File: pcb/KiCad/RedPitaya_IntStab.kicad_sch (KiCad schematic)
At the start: 28 parts, among them J1 C64AC, J16 Hold_2, J4 Hold_1

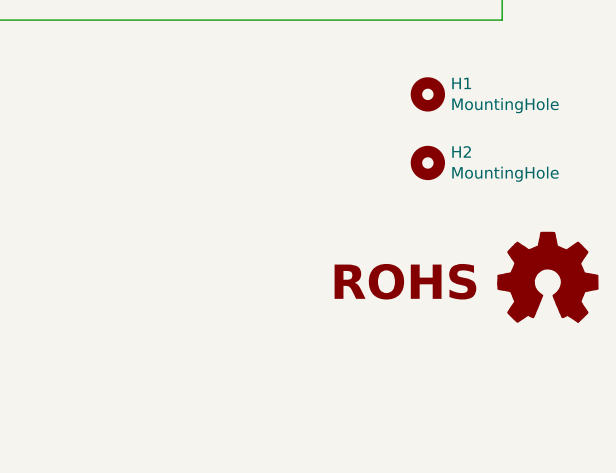
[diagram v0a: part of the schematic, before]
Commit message: More logo updates
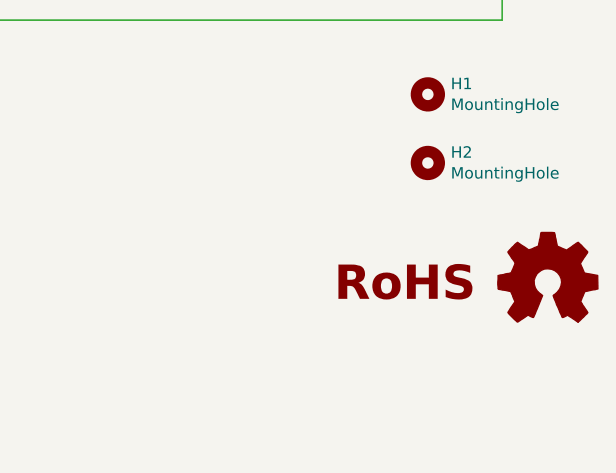
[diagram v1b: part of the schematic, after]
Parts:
- LOGO1, LOGO3: now left out of the parts list
- LOGO2: value Logo_ROHS -> Logo_RoHS; symbol Custom_logos:Logo_ROHS -> Custom_logos:Logo_RoHS; now left out of the parts list
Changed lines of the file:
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@@
   )
   (symbol (lib_id "Custom_logos:Logo_APQ") (at 173.99 171.45 0) (unit 1)
-    (in_bom yes) (on_board yes) (dnp no)
+    (in_bom no) (on_board yes) (dnp no)
     (property "Reference" "LOGO1" (at 180.34 164.465 0)
       (effects (font (size 1.27 1.27)) hide)
@@
       (effects (font (size 1.27 1.27)) hide)
     )
+    (property "MFN" "" (at 173.99 171.45 0)
+      (effects (font (size 1.27 1.27)) hide)
+    )
+    (property "PN" "" (at 173.99 171.45 0)
+      (effects (font (size 1.27 1.27)) hide)
+    )
+    (property "Sim.Enable" "0" (at 173.99 171.45 0)
+      (effects (font (size 1.27 1.27)) hide)
+    )
     (instances
       (project "RedPitaya_IntStab"
@@
   )
   (symbol (lib_id "Graphic:Logo_Open_Hardware_Small") (at 278.13 172.72 0) (unit 1)
-    (in_bom yes) (on_board yes) (dnp no)
+    (in_bom no) (on_board yes) (dnp no)
     (property "Reference" "LOGO3" (at 278.13 165.735 0)
       (effects (font (size 1.27 1.27)) hide)
@@
       (effects (font (size 1.27 1.27)) hide)
     )
+    (property "MFN" "" (at 278.13 172.72 0)
+      (effects (font (size 1.27 1.27)) hide)
+    )
+    (property "PN" "" (at 278.13 172.72 0)
+      (effects (font (size 1.27 1.27)) hide)
+    )
+    (property "Sim.Enable" "0" (at 278.13 172.72 0)
+      (effects (font (size 1.27 1.27)) hide)
+    )
     (instances
       (project "RedPitaya_IntStab"
@@
     )
   )
-  (symbol (lib_id "Custom_logos:Logo_ROHS") (at 248.92 172.72 0) (unit 1)
-    (in_bom yes) (on_board yes) (dnp no)
+  (symbol (lib_id "Custom_logos:Logo_RoHS") (at 248.92 172.72 0) (unit 1)
+    (in_bom no) (on_board yes) (dnp no)
     (property "Reference" "LOGO2" (at 255.27 165.735 0)
       (effects (font (size 1.27 1.27)) hide)
     )
-    (property "Value" "Logo_ROHS" (at 255.27 179.07 0)
+    (property "Value" "Logo_RoHS" (at 255.27 179.07 0)
       (effects (font (size 1.27 1.27)) hide)
     )
-    (property "Footprint" "Symbol:RoHS-Logo_6mm_SilkScreen" (at 262.255 168.1734 0)
+    (property "Footprint" "Symbol:RoHS-Logo_6mm_SilkScreen" (at 256.54 172.72 0)
       (effects (font (size 1.27 1.27)) hide)
     )
@@
       (effects (font (size 1.27 1.27)) hide)
     )
+    (property "MFN" "" (at 248.92 172.72 0)
+      (effects (font (size 1.27 1.27)) hide)
+    )
+    (property "PN" "" (at 248.92 172.72 0)
+      (effects (font (size 1.27 1.27)) hide)
+    )
+    (property "Sim.Enable" "0" (at 248.92 172.72 0)
+      (effects (font (size 1.27 1.27)) hide)
+    )

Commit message: Fixed solder jumpers
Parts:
- JP10, JP11, JP12, JP13, JP14, JP15, JP3, JP4, JP5, JP6, JP7, JP8, JP9: footprint Jumper:SolderJumper-2_P1.3mm_Open_RoundedPad1.0x1.5mm -> Jumper:SolderJumper-2_P1.3mm_Bridged_RoundedPad1.0x1.5mm
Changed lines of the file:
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@@
       (effects (font (size 1.27 1.27)))
     )
-    (property "Footprint" "Jumper:SolderJumper-2_P1.3mm_Open_RoundedPad1.0x1.5mm" (at 19.05 171.45 0)
+    (property "Footprint" "Jumper:SolderJumper-2_P1.3mm_Bridged_RoundedPad1.0x1.5mm" (at 19.05 171.45 0)
       (effects (font (size 1.27 1.27)) hide)
     )
@@
       (effects (font (size 1.27 1.27)) hide)
     )
+    (property "MFN" "" (at 19.05 171.45 0)
+      (effects (font (size 1.27 1.27)) hide)
+    )
+    (property "PN" "" (at 19.05 171.45 0)
+      (effects (font (size 1.27 1.27)) hide)
+    )
     (pin "1")
     (pin "2")
@@
       (effects (font (size 1.27 1.27)))
     )
-    (property "Footprint" "Jumper:SolderJumper-2_P1.3mm_Open_RoundedPad1.0x1.5mm" (at 49.53 187.96 0)
+    (property "Footprint" "Jumper:SolderJumper-2_P1.3mm_Bridged_RoundedPad1.0x1.5mm" (at 49.53 187.96 0)
       (effects (font (size 1.27 1.27)) hide)
     )
@@
       (effects (font (size 1.27 1.27)) hide)
     )
+    (property "MFN" "" (at 49.53 187.96 0)
+      (effects (font (size 1.27 1.27)) hide)
+    )
+    (property "PN" "" (at 49.53 187.96 0)
+      (effects (font (size 1.27 1.27)) hide)
+    )
     (pin "1")
     (pin "2")
@@
       (effects (font (size 1.27 1.27)))
     )
-    (property "Footprint" "Jumper:SolderJumper-2_P1.3mm_Open_RoundedPad1.0x1.5mm" (at 19.05 144.78 0)
+    (property "Footprint" "Jumper:SolderJumper-2_P1.3mm_Bridged_RoundedPad1.0x1.5mm" (at 19.05 144.78 0)
       (effects (font (size 1.27 1.27)) hide)
     )
@@
       (effects (font (size 1.27 1.27)) hide)
     )
+    (property "MFN" "" (at 19.05 144.78 0)
+      (effects (font (size 1.27 1.27)) hide)
+    )
+    (property "PN" "" (at 19.05 144.78 0)
+      (effects (font (size 1.27 1.27)) hide)
+    )
     (pin "1")
     (pin "2")
@@
       (effects (font (size 1.27 1.27)))
     )
-    (property "Footprint" "Jumper:SolderJumper-2_P1.3mm_Open_RoundedPad1.0x1.5mm" (at 19.05 129.54 0)
+    (property "Footprint" "Jumper:SolderJumper-2_P1.3mm_Bridged_RoundedPad1.0x1.5mm" (at 19.05 129.54 0)
       (effects (font (size 1.27 1.27)) hide)
     )
@@
       (effects (font (size 1.27 1.27)) hide)
     )
+    (property "MFN" "" (at 19.05 129.54 0)
+      (effects (font (size 1.27 1.27)) hide)
+    )
+    (property "PN" "" (at 19.05 129.54 0)
+      (effects (font (size 1.27 1.27)) hide)
+    )
     (pin "1")
     (pin "2")
@@
       (effects (font (size 1.27 1.27)))
     )
-    (property "Footprint" "Jumper:SolderJumper-2_P1.3mm_Open_RoundedPad1.0x1.5mm" (at 50.8 133.35 0)
+    (property "Footprint" "Jumper:SolderJumper-2_P1.3mm_Bridged_RoundedPad1.0x1.5mm" (at 50.8 133.35 0)
       (effects (font (size 1.27 1.27)) hide)
     )
@@
       (effects (font (size 1.27 1.27)) hide)
     )
+    (property "MFN" "" (at 50.8 133.35 0)
+      (effects (font (size 1.27 1.27)) hide)
+    )
+    (property "PN" "" (at 50.8 133.35 0)
+      (effects (font (size 1.27 1.27)) hide)
+    )
     (pin "1")
     (pin "2")
@@
       (effects (font (size 1.27 1.27)))
     )
-    (property "Footprint" "Jumper:SolderJumper-2_P1.3mm_Open_RoundedPad1.0x1.5mm" (at 19.05 180.34 0)
+    (property "Footprint" "Jumper:SolderJumper-2_P1.3mm_Bridged_RoundedPad1.0x1.5mm" (at 19.05 180.34 0)
       (effects (font (size 1.27 1.27)) hide)
     )
@@
       (effects (font (size 1.27 1.27)) hide)
     )
+    (property "MFN" "" (at 19.05 180.34 0)
+      (effects (font (size 1.27 1.27)) hide)
+    )
+    (property "PN" "" (at 19.05 180.34 0)
+      (effects (font (size 1.27 1.27)) hide)
+    )
     (pin "1")
     (pin "2")
@@
       (effects (font (size 1.27 1.27)))
     )
-    (property "Footprint" "Jumper:SolderJumper-2_P1.3mm_Open_RoundedPad1.0x1.5mm" (at 50.8 124.46 0)
+    (property "Footprint" "Jumper:SolderJumper-2_P1.3mm_Bridged_RoundedPad1.0x1.5mm" (at 50.8 124.46 0)
       (effects (font (size 1.27 1.27)) hide)
     )
@@
       (effects (font (size 1.27 1.27)) hide)
     )
+    (property "MFN" "" (at 50.8 124.46 0)
+      (effects (font (size 1.27 1.27)) hide)
+    )
+    (property "PN" "" (at 50.8 124.46 0)
+      (effects (font (size 1.27 1.27)) hide)
+    )
     (pin "1")
     (pin "2")
@@
       (effects (font (size 1.27 1.27)))
     )
-    (property "Footprint" "Jumper:SolderJumper-2_P1.3mm_Open_RoundedPad1.0x1.5mm" (at 19.05 137.16 0)
+    (property "Footprint" "Jumper:SolderJumper-2_P1.3mm_Bridged_RoundedPad1.0x1.5mm" (at 19.05 137.16 0)
       (effects (font (size 1.27 1.27)) hide)
     )
@@
       (effects (font (size 1.27 1.27)) hide)
     )
+    (property "MFN" "" (at 19.05 137.16 0)
+      (effects (font (size 1.27 1.27)) hide)
+    )
+    (property "PN" "" (at 19.05 137.16 0)
+      (effects (font (size 1.27 1.27)) hide)
+    )
     (pin "1")
     (pin "2")
@@
       (effects (font (size 1.27 1.27)))
     )
-    (property "Footprint" "Jumper:SolderJumper-2_P1.3mm_Open_RoundedPad1.0x1.5mm" (at 19.05 153.67 0)
+    (property "Footprint" "Jumper:SolderJumper-2_P1.3mm_Bridged_RoundedPad1.0x1.5mm" (at 19.05 153.67 0)
       (effects (font (size 1.27 1.27)) hide)
     )
@@
     )
     (property "Config" "DNF" (at 19.05 153.67 0)
+      (effects (font (size 1.27 1.27)) hide)
+    )
+    (property "MFN" "" (at 19.05 153.67 0)
+      (effects (font (size 1.27 1.27)) hide)
+    )
+    (property "PN" "" (at 19.05 153.67 0)
       (effects (font (size 1.27 1.27)) hide)
     )
@@
       (effects (font (size 1.27 1.27)))
     )
-    (property "Footprint" "Jumper:SolderJumper-2_P1.3mm_Open_RoundedPad1.0x1.5mm" (at 49.53 171.45 0)
+    (property "Footprint" "Jumper:SolderJumper-2_P1.3mm_Bridged_RoundedPad1.0x1.5mm" (at 49.53 171.45 0)
       (effects (font (size 1.27 1.27)) hide)
     )
@@
       (effects (font (size 1.27 1.27)) hide)
     )
+    (property "MFN" "" (at 49.53 171.45 0)
+      (effects (font (size 1.27 1.27)) hide)
+    )
+    (property "PN" "" (at 49.53 171.45 0)
+      (effects (font (size 1.27 1.27)) hide)
+    )
     (pin "1")
     (pin "2")
@@
       (effects (font (size 1.27 1.27)))
     )
-    (property "Footprint" "Jumper:SolderJumper-2_P1.3mm_Open_RoundedPad1.0x1.5mm" (at 19.05 121.92 0)
+    (property "Footprint" "Jumper:SolderJumper-2_P1.3mm_Bridged_RoundedPad1.0x1.5mm" (at 19.05 121.92 0)
       (effects (font (size 1.27 1.27)) hide)
     )
@@
       (effects (font (size 1.27 1.27)) hide)
     )
+    (property "MFN" "" (at 19.05 121.92 0)
+      (effects (font (size 1.27 1.27)) hide)
+    )
+    (property "PN" "" (at 19.05 121.92 0)
+      (effects (font (size 1.27 1.27)) hide)
+    )
     (pin "1")
     (pin "2")
@@
       (effects (font (size 1.27 1.27)))
     )
-    (property "Footprint" "Jumper:SolderJumper-2_P1.3mm_Open_RoundedPad1.0x1.5mm" (at 19.05 162.56 0)
+    (property "Footprint" "Jumper:SolderJumper-2_P1.3mm_Bridged_RoundedPad1.0x1.5mm" (at 19.05 162.56 0)
       (effects (font (size 1.27 1.27)) hide)
     )
@@
       (effects (font (size 1.27 1.27)) hide)
     )
+    (property "MFN" "" (at 19.05 162.56 0)
+      (effects (font (size 1.27 1.27)) hide)
+    )
+    (property "PN" "" (at 19.05 162.56 0)
+      (effects (font (size 1.27 1.27)) hide)
+    )
     (pin "1")
     (pin "2")
@@
       (effects (font (size 1.27 1.27)))
     )
-    (property "Footprint" "Jumper:SolderJumper-2_P1.3mm_Open_RoundedPad1.0x1.5mm" (at 50.8 116.84 0)
+    (property "Footprint" "Jumper:SolderJumper-2_P1.3mm_Bridged_RoundedPad1.0x1.5mm" (at 50.8 116.84 0)
       (effects (font (size 1.27 1.27)) hide)
     )
@@
       (effects (font (size 1.27 1.27)) hide)
     )
+    (property "MFN" "" (at 50.8 116.84 0)
+      (effects (font (size 1.27 1.27)) hide)
+    )
+    (property "PN" "" (at 50.8 116.84 0)
+      (effects (font (size 1.27 1.27)) hide)
+    )

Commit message: Fixed logos on the schematic
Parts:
- LOGO1, LOGO2, LOGO3: Config DNF -> (none)
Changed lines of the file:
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@@
-      (effects (font (size 1.27 1.27)) hide)
-    )
-    (property "Config" "DNF" (at 173.99 171.45 0)
       (effects (font (size 1.27 1.27)) hide)
     )
@@
       (effects (font (size 1.27 1.27)) hide)
     )
-    (property "Config" "DNF" (at 278.13 172.72 0)
-      (effects (font (size 1.27 1.27)) hide)
-    )
     (property "MFN" "" (at 278.13 172.72 0)
       (effects (font (size 1.27 1.27)) hide)
@@
       (effects (font (size 1.27 1.27)) hide)
     )
-    (property "Config" "DNF" (at 248.92 172.72 0)
-      (effects (font (size 1.27 1.27)) hide)
-    )
